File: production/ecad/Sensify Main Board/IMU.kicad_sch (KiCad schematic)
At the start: 5 parts, among them U5 LSM6DSOTR

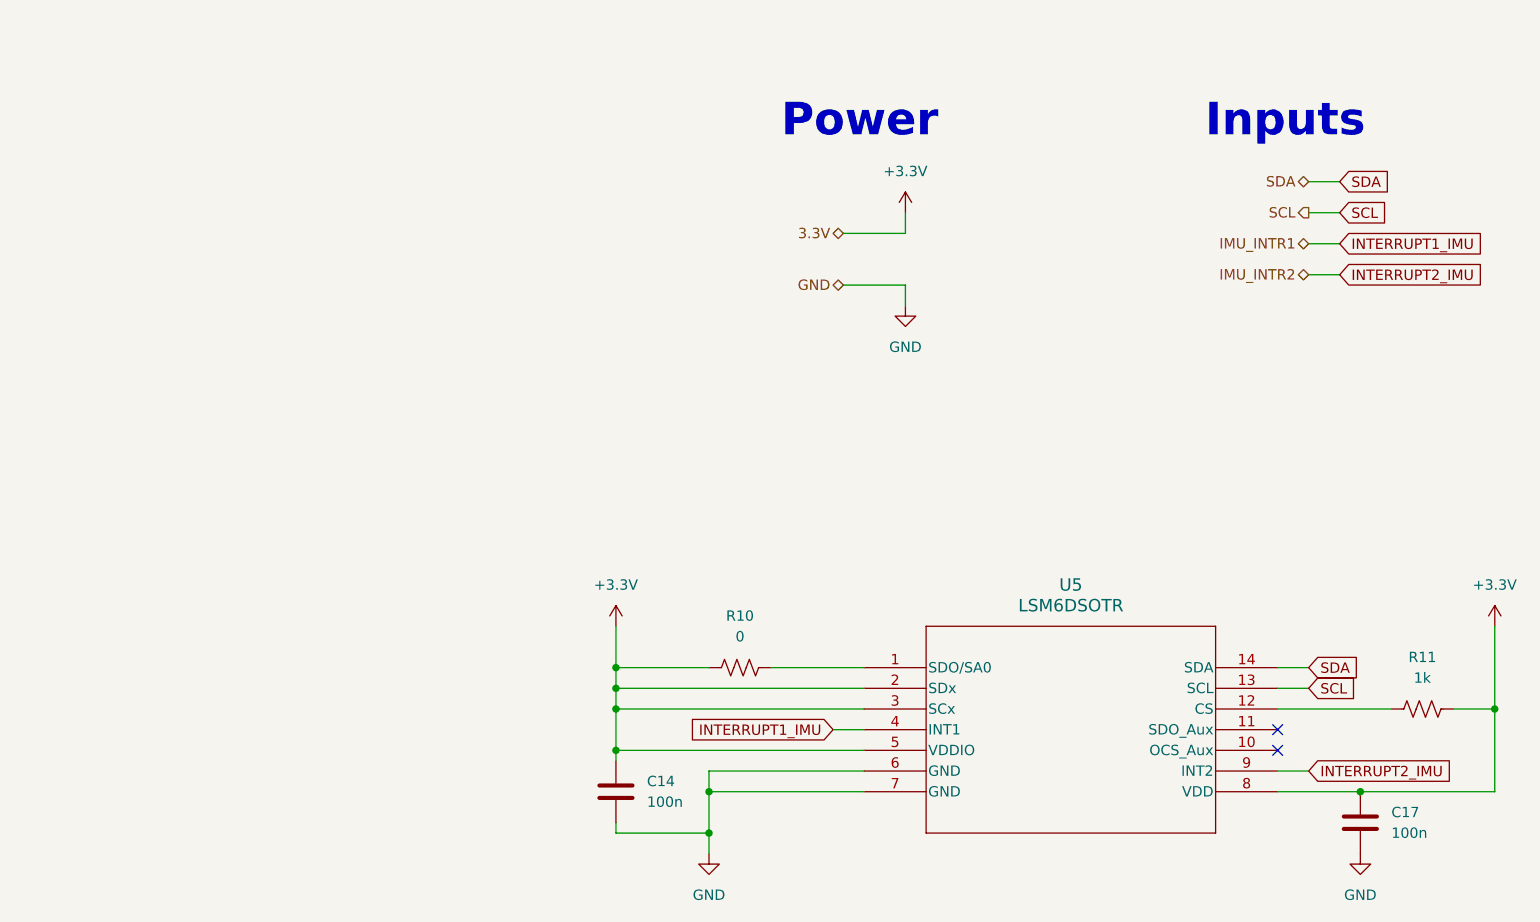
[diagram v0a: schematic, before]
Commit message: Finished IMU, Haptics, MCU, and Root Page
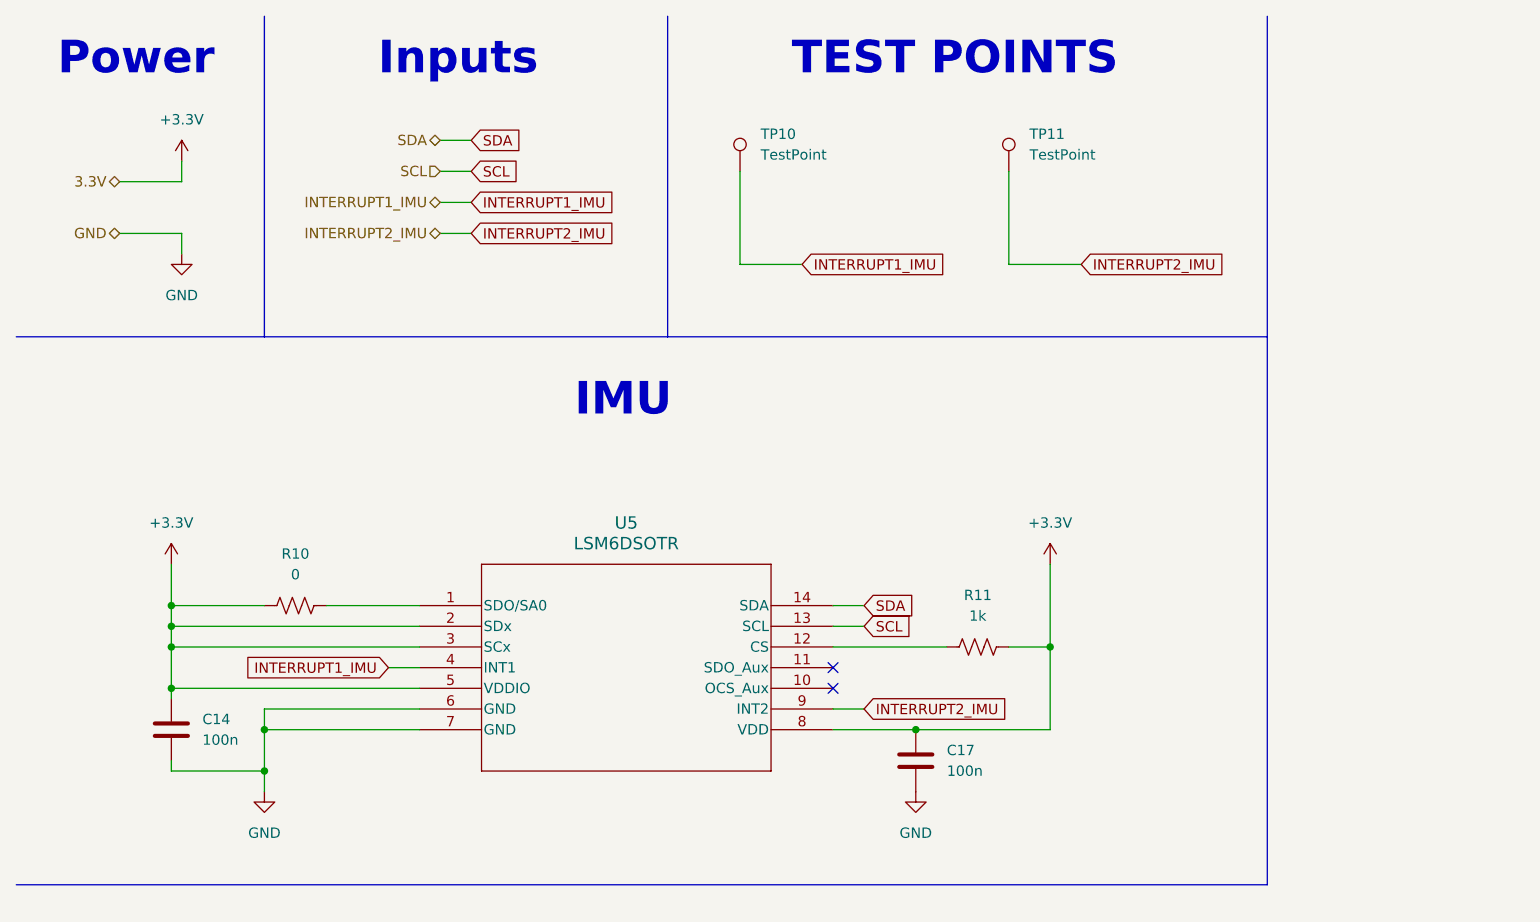
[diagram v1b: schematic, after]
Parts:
- added TP10, TP11: TestPoint, symbol Connector:TestPoint
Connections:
- net INTERRUPT1_IMU: now also TP10.1
- net INTERRUPT2_IMU: now also TP11.1
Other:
- note added: "IMU"
- note added: "TEST POINTS"
- moved on the sheet: C14, C17, R10, R11, U5
